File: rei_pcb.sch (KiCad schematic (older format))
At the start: 163 parts, among them J1 SM04B-SRSS-TB(LF)(SN), SW1 SW_Push, U2 ATmega32U4RC-MU, Y1 16MHz

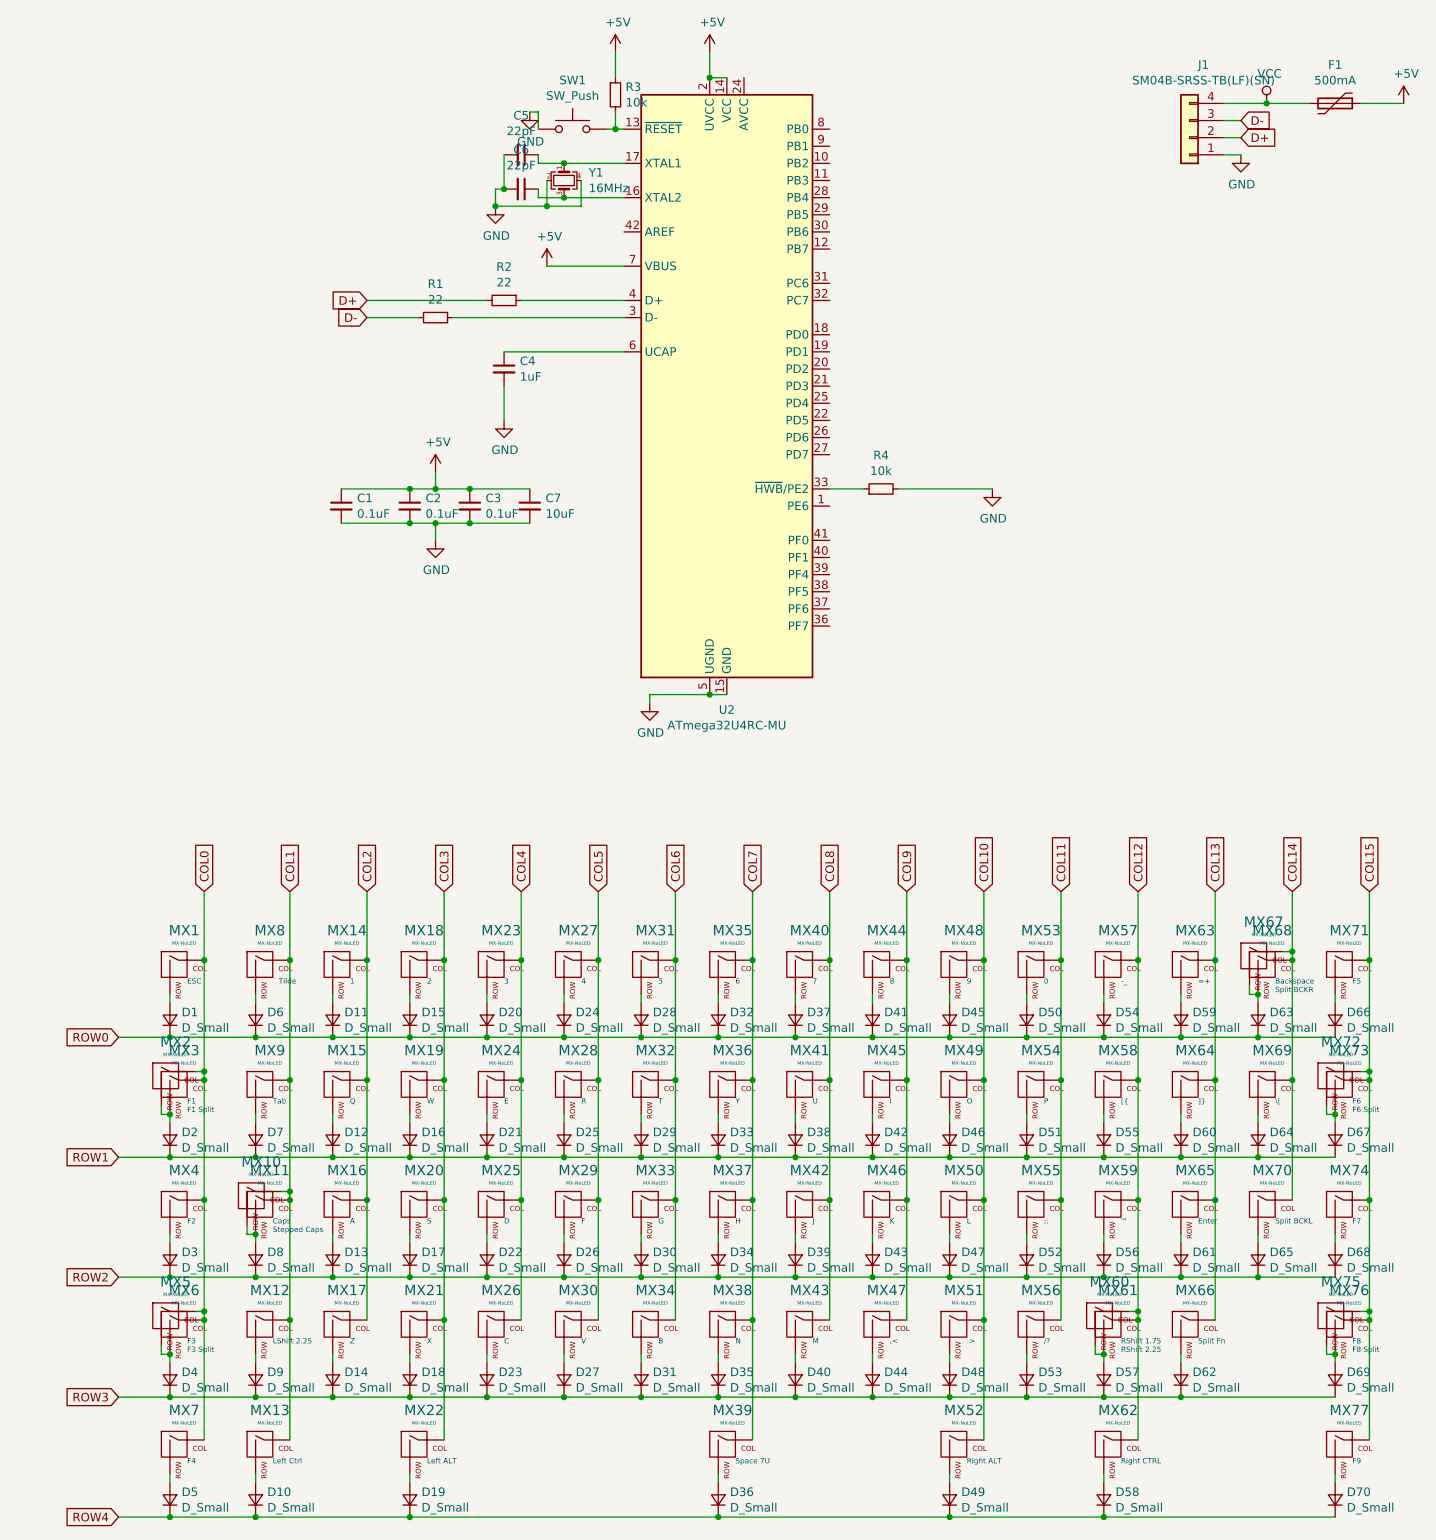
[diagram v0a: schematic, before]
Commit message: PCB initial complete
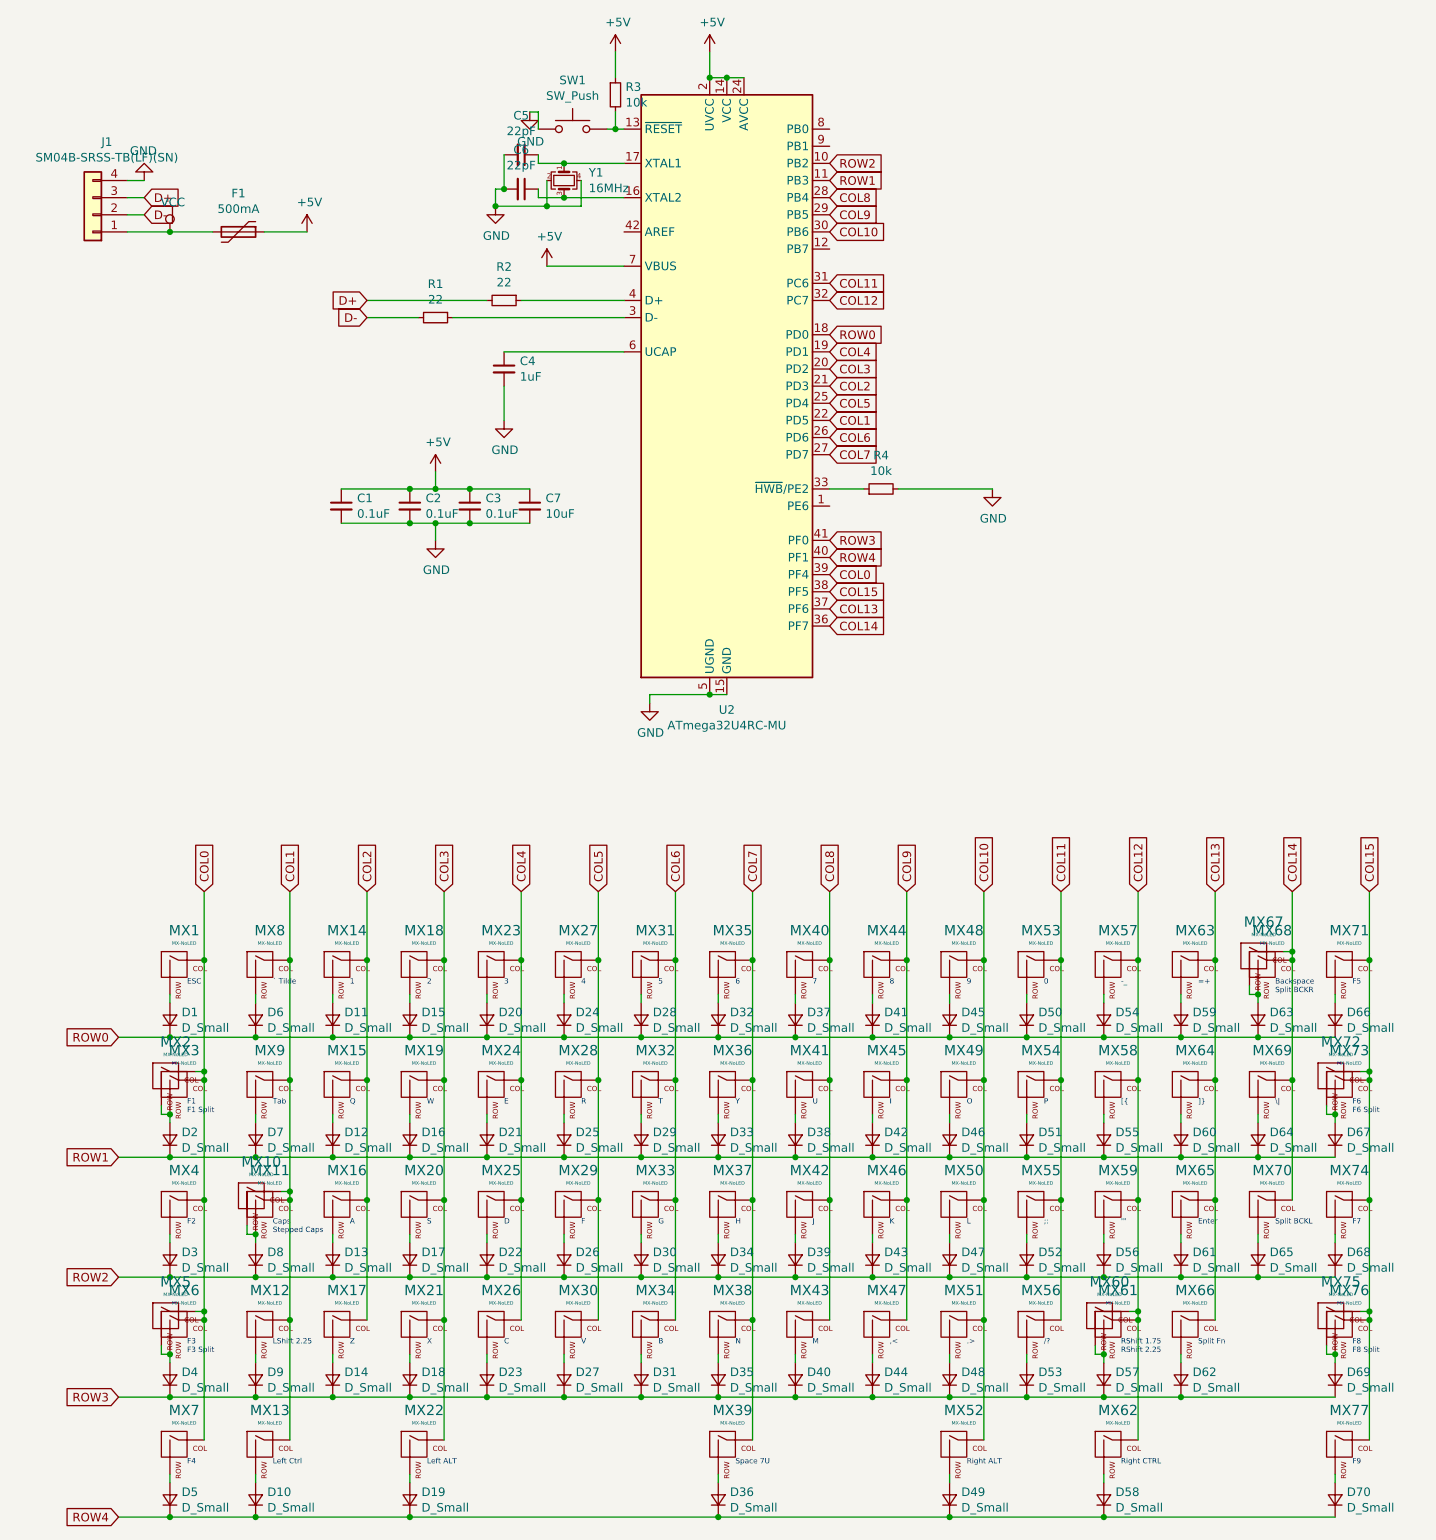
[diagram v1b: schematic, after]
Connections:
- net +5V: now also U2.24 (AVCC), U2.44 (AVCC)
- net COL0: now also U2.39 (PF4)
- net COL1: now also U2.22 (PD5)
- net COL10: now also U2.30 (PB6)
- net COL11: now also U2.31 (PC6)
- net COL12: now also U2.32 (PC7)
- net COL13: now also U2.37 (PF6)
- net COL14: now also U2.36 (PF7)
- net COL15: now also U2.38 (PF5)
- net COL2: now also U2.21 (PD3)
- net COL3: now also U2.20 (PD2)
- net COL4: now also U2.19 (PD1)
- net COL5: now also U2.25 (PD4)
- net COL6: now also U2.26 (PD6)
- net COL7: now also U2.27 (PD7)
- net COL8: now also U2.28 (PB4)
- net COL9: now also U2.29 (PB5)
- net D+: now also J1.3 (Pin_3); no longer J1.2 (Pin_2)
- net D-: now also J1.2 (Pin_2); no longer J1.3 (Pin_3)
- net GND: now also J1.4 (Pin_4); no longer J1.1 (Pin_1)
- net ROW0: now also U2.18 (PD0)
- net ROW1: now also U2.11 (PB3)
- net ROW2: now also U2.10 (PB2)
- net ROW3: now also U2.41 (PF0)
- net ROW4: now also U2.40 (PF1)
- net VCC: now also J1.1 (Pin_1); no longer J1.4 (Pin_4)
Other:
- moved on the sheet: F1, J1
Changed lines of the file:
@@
 L power:VCC #PWR012
 U 1 1 5EA86CA0
-P 9900 1650
-F 0 "#PWR012" H 9900 1500 50  0001 C CNN
-F 1 "VCC" H 9917 1823 50  0000 C CNN
-F 2 "" H 9900 1650 50  0001 C CNN
-F 3 "" H 9900 1650 50  0001 C CNN
-	1    9900 1650
+P 3500 2400
+F 0 "#PWR012" H 3500 2250 50  0001 C CNN
+F 1 "VCC" H 3517 2573 50  0000 C CNN
+F 2 "" H 3500 2400 50  0001 C CNN
+F 3 "" H 3500 2400 50  0001 C CNN
+	1    3500 2400
 	1    0    0    -1
 $EndComp
@@
 L Device:Polyfuse F1
 U 1 1 5EA87A4A
-P 10300 1650
-F 0 "F1" V 10075 1650 50  0000 C CNN
-F 1 "500mA" V 10166 1650 50  0000 C CNN
-F 2 "Fuse:Fuse_1206_3216Metric" H 10350 1450 50  0001 L CNN
-F 3 "~" H 10300 1650 50  0001 C CNN
-	1    10300 1650
+P 3900 2400
+F 0 "F1" V 3675 2400 50  0000 C CNN
+F 1 "500mA" V 3766 2400 50  0000 C CNN
+F 2 "Fuse:Fuse_1206_3216Metric" H 3950 2200 50  0001 L CNN
+F 3 "~" H 3900 2400 50  0001 C CNN
+	1    3900 2400
 	0    1    1    0
 $EndComp
@@
 L power:+5V #PWR013
 U 1 1 5EA88909
-P 10700 1650
-F 0 "#PWR013" H 10700 1500 50  0001 C CNN
-F 1 "+5V" H 10715 1823 50  0000 C CNN
-F 2 "" H 10700 1650 50  0001 C CNN
-F 3 "" H 10700 1650 50  0001 C CNN
-	1    10700 1650
-	1    0    0    -1
-$EndComp
-Wire Wire Line
-	10700 1650 10450 1650
-Wire Wire Line
-	10150 1650 9900 1650
-Connection ~ 9900 1650
-Wire Wire Line
-	9900 1650 9650 1650
-Text GLabel 9750 1750 2    50   Input ~ 0
+P 4300 2400
+F 0 "#PWR013" H 4300 2250 50  0001 C CNN
+F 1 "+5V" H 4315 2573 50  0000 C CNN
+F 2 "" H 4300 2400 50  0001 C CNN
+F 3 "" H 4300 2400 50  0001 C CNN
+	1    4300 2400
+	1    0    0    -1
+$EndComp
+Wire Wire Line
+	4300 2400 4050 2400
+Wire Wire Line
+	3750 2400 3500 2400
+Connection ~ 3500 2400
+Wire Wire Line
+	3500 2400 3250 2400
+Text GLabel 3350 2300 2    50   Input ~ 0
 D-
-Text GLabel 9750 1850 2    50   Input ~ 0
+Text GLabel 3350 2200 2    50   Input ~ 0
 D+
 $Comp
 L power:GND #PWR011
 U 1 1 5EA8EB87
-P 9750 1950
-F 0 "#PWR011" H 9750 1700 50  0001 C CNN
-F 1 "GND" H 9755 1777 50  0000 C CNN
-F 2 "" H 9750 1950 50  0001 C CNN
-F 3 "" H 9750 1950 50  0001 C CNN
-	1    9750 1950
-	1    0    0    -1
-$EndComp
-Wire Wire Line
-	9750 1850 9650 1850
-Wire Wire Line
-	9650 1750 9750 1750
+P 3350 2100
+F 0 "#PWR011" H 3350 1850 50  0001 C CNN
+F 1 "GND" H 3355 1927 50  0000 C CNN
+F 2 "" H 3350 2100 50  0001 C CNN
+F 3 "" H 3350 2100 50  0001 C CNN
+	1    3350 2100
+	-1   0    0    1
+$EndComp
+Wire Wire Line
+	3350 2200 3250 2200
+Wire Wire Line
+	3250 2300 3350 2300
 $Comp
 L MX_Alps_Hybrid:MX-NoLED MX1
@@
 L Connector_Generic:Conn_01x04 J1
 U 1 1 5EA8BBC7
-P 9450 1850
-F 0 "J1" H 9368 1425 50  0000 C CNN
-F 1 "SM04B-SRSS-TB(LF)(SN)" H 9368 1516 50  0000 C CNN
-F 2 "random-keyboard-parts:JST-SR-4" H 9450 1850 50  0001 C CNN
-F 3 "~" H 9450 1850 50  0001 C CNN
-	1    9450 1850
+P 3050 2300
+F 0 "J1" H 2968 1875 50  0000 C CNN
+F 1 "SM04B-SRSS-TB(LF)(SN)" H 2968 1966 50  0000 C CNN
+F 2 "random-keyboard-parts:JST-SR-4" H 3050 2300 50  0001 C CNN
+F 3 "~" H 3050 2300 50  0001 C CNN
+	1    3050 2300
 	-1   0    0    1
 $EndComp
 Wire Wire Line
-	9650 1950 9750 1950
+	3250 2100 3350 2100
 Wire Wire Line
 	10300 8250 10300 8300
@@
 	6750 5100 6650 5100
 Connection ~ 6650 5100
+Wire Wire Line
+	6850 1500 6750 1500
+Connection ~ 6750 1500
+Text GLabel 7350 4400 2    50   Input ~ 0
+COL0
+Text GLabel 7350 3500 2    50   Input ~ 0
+COL1
+Text GLabel 7350 3300 2    50   Input ~ 0
+COL2
+Text GLabel 7350 3200 2    50   Input ~ 0
+COL3
+Text GLabel 7350 3100 2    50   Input ~ 0
+COL4
+Text GLabel 7350 3400 2    50   Input ~ 0
+COL5
+Text GLabel 7350 3600 2    50   Input ~ 0
+COL6
+Text GLabel 7350 3700 2    50   Input ~ 0
+COL7
+Text GLabel 7350 2200 2    50   Input ~ 0
+COL8
+Text GLabel 7350 2300 2    50   Input ~ 0
+COL9
+Text GLabel 7350 2400 2    50   Input ~ 0
+COL10
+Text GLabel 7350 2700 2    50   Input ~ 0
+COL11
+Text GLabel 7350 2800 2    50   Input ~ 0
+COL12
+Text GLabel 7350 4600 2    50   Input ~ 0
+COL13
+Text GLabel 7350 3000 2    50   Input ~ 0
+ROW0
+Text GLabel 7350 2000 2    50   Input ~ 0
+ROW2
+Text GLabel 7350 2100 2    50   Input ~ 0
+ROW1
+Text GLabel 7350 4200 2    50   Input ~ 0
+ROW3
+Text GLabel 7350 4300 2    50   Input ~ 0
+ROW4
+Text GLabel 7350 4700 2    50   Input ~ 0
+COL14
+Text GLabel 7350 4500 2    50   Input ~ 0
+COL15
 $EndSCHEMATC

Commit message: Completed PCB
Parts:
- MX3, MX6, MX73, MX76: footprint MX_Only:MXOnly-2U-FLIPPED -> MX_Only:MXOnly-2U-NoLED
- MX65: footprint MX_Only:MXOnly-2.25U-FLIPPED-ReversedStabilizers -> MX_Only:MXOnly-2.25U-ReversedStabilizers-NoLED
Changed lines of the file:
@@
 F 0 "MX3" H 3583 7623 60  0000 C CNN
 F 1 "MX-NoLED" H 3583 7549 20  0000 C CNN
-F 2 "MX_Only:MXOnly-2U-FLIPPED" H 2925 7375 60  0001 C CNN
+F 2 "MX_Only:MXOnly-2U-NoLED" H 2925 7375 60  0001 C CNN
 F 3 "" H 2925 7375 60  0001 C CNN
 	1    3550 7400
@@
 F 0 "MX6" H 3583 9023 60  0000 C CNN
 F 1 "MX-NoLED" H 3583 8949 20  0000 C CNN
-F 2 "MX_Only:MXOnly-2U-FLIPPED" H 2925 8775 60  0001 C CNN
+F 2 "MX_Only:MXOnly-2U-NoLED" H 2925 8775 60  0001 C CNN
 F 3 "" H 2925 8775 60  0001 C CNN
 	1    3550 8800
@@
 F 0 "MX65" H 9483 8323 60  0000 C CNN
 F 1 "MX-NoLED" H 9483 8249 20  0000 C CNN
-F 2 "MX_Only:MXOnly-2.25U-FLIPPED-ReversedStabilizers" H 8825 8075 60  0001 C CNN
+F 2 "MX_Only:MXOnly-2.25U-ReversedStabilizers-NoLED" H 8825 8075 60  0001 C CNN
 F 3 "" H 8825 8075 60  0001 C CNN
 	1    9450 8100
@@
 F 0 "MX73" H 10383 7623 60  0000 C CNN
 F 1 "MX-NoLED" H 10383 7549 20  0000 C CNN
-F 2 "MX_Only:MXOnly-2U-FLIPPED" H 9725 7375 60  0001 C CNN
+F 2 "MX_Only:MXOnly-2U-NoLED" H 9725 7375 60  0001 C CNN
 F 3 "" H 9725 7375 60  0001 C CNN
 	1    10350 7400
@@
 F 0 "MX76" H 10383 9023 60  0000 C CNN
 F 1 "MX-NoLED" H 10383 8949 20  0000 C CNN
-F 2 "MX_Only:MXOnly-2U-FLIPPED" H 9725 8775 60  0001 C CNN
+F 2 "MX_Only:MXOnly-2U-NoLED" H 9725 8775 60  0001 C CNN
 F 3 "" H 9725 8775 60  0001 C CNN
 	1    10350 8800
